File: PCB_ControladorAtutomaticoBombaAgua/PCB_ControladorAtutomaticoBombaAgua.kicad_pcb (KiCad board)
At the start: 4 copper layers, 78 x 57 mm, 20 parts, among them J1 Sensor, K1 Relay12V, K2 Relay12V, P1 12V, P2 230VAC/50Hz, P3 Motor/Bomba, Q1 BC547, Q2 BC547, Q3 BC547, U1 CD4011

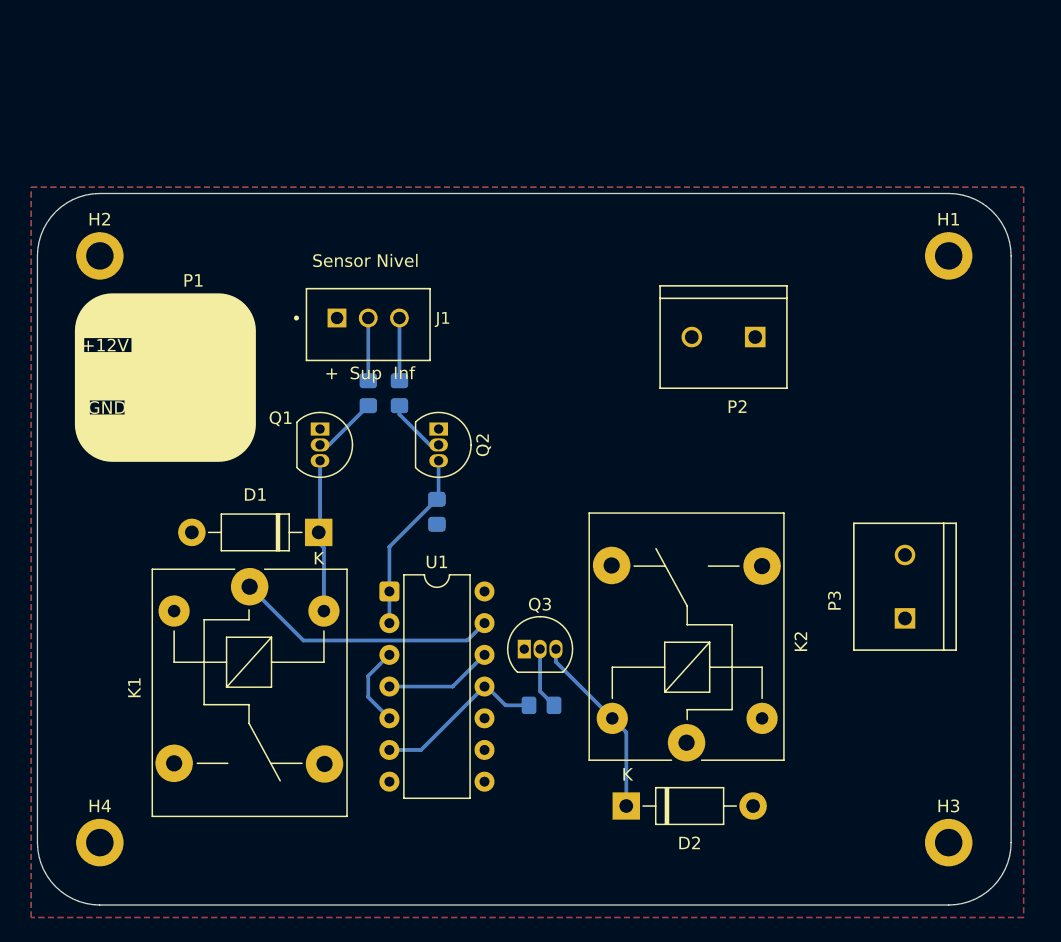
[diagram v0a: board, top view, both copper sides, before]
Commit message: Finalizado
Diseño completado
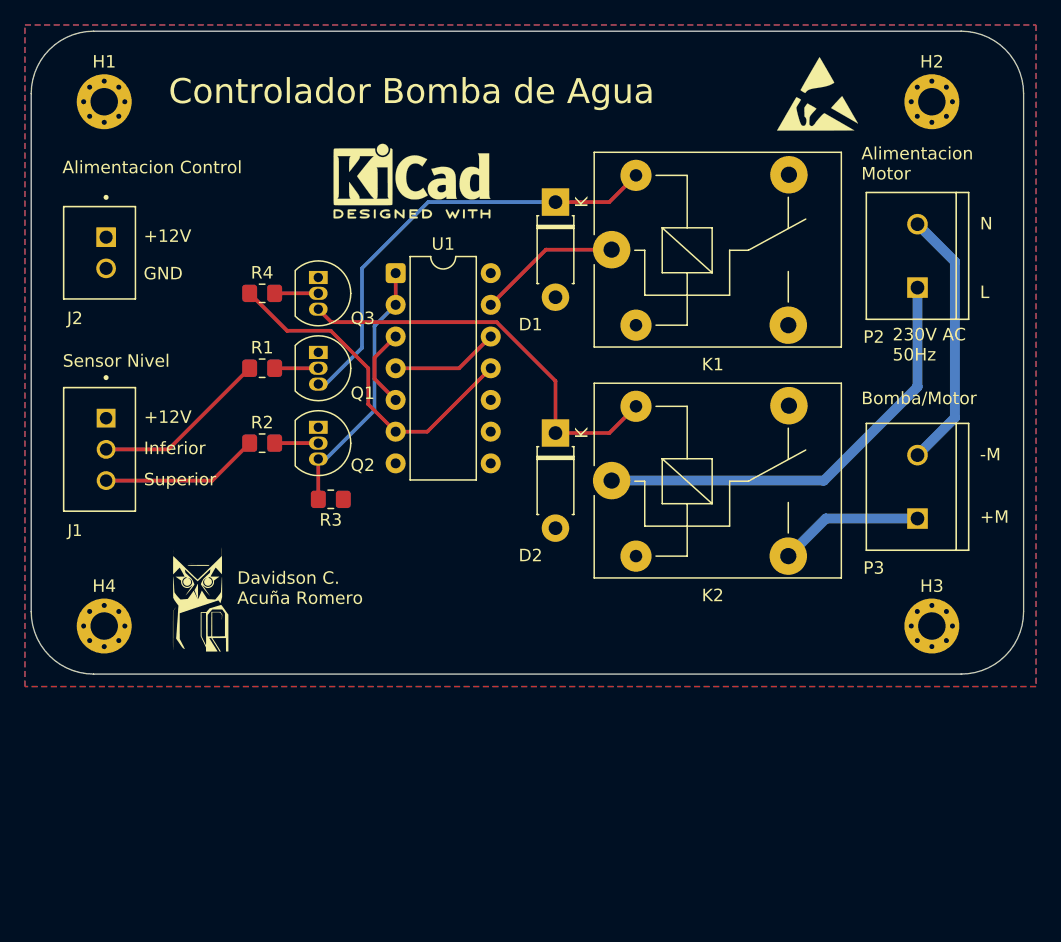
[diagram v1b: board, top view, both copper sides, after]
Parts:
- removed P1: 12V, BORNERA_2:BORNERA-2
- added G***: LOGO, SHIFT:Buho_10X10mm, F.Cu at (135.5, 88.5)
- added G***: LOGO, Huellas:Sensor16x20, B.Cu at (137.0, 66.0)
- added J2: Alimen/Control, JST_XH_2:JST_B2B-XH-A, F.Cu at (127.5, 60.8)
- added REF**: ESD-Logo_6.6x6mm_SilkScreen, Symbol:ESD-Logo_6.6x6mm_SilkScreen, F.Cu at (185.0, 48.0)
- added REF**: KiCad-Logo2_5mm_SilkScreen, Symbol:KiCad-Logo2_5mm_SilkScreen, F.Cu at (152.5, 55.0)
- D1, D2: footprint Diode_THT:D_DO-41_SOD81_P10.16mm_Horizontal -> Diode_THT:D_DO-41_SOD81_P7.62mm_Horizontal
- H1, H2, H3, H4: footprint MountingHole:MountingHole_2.2mm_M2_DIN965_Pad -> MountingHole:MountingHole_2.2mm_M2_Pad_Via
- R1, R2, R3, R4: moved to F.Cu
- moved H1 68.8 mm to (127.8, 48.6)
- moved H2 67.8 mm to (194.2, 48.6)
- moved R4 39.9 mm to (140.5, 64.0)
- moved K1 39.6 mm to (168.5, 60.5), turned to 0 degrees
- moved Q3 34.0 mm to (145.0, 62.7), turned to -90 degrees
- moved D1 32.6 mm to (164.0, 56.7), turned to -90 degrees
- moved D2 30.4 mm to (164.0, 75.2), turned to -90 degrees
- moved U1 25.5 mm to (151.2, 62.4)
- moved J1 23.7 mm to (127.5, 76.5), turned to 90 degrees
- moved K2 21.8 mm to (168.5, 79.0), turned to 0 degrees
- moved H3 17.4 mm to (194.2, 90.7)
- moved H4 17.4 mm to (127.8, 90.7)
- moved P2 16.8 mm to (193.0, 61.0), turned to 90 degrees
- moved R2 11.7 mm to (140.5, 76.0), turned to 0 degrees
- moved Q2 9.64 mm to (145.0, 74.7)
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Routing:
- net LINE: track 0.00 -> 35.6 mm
- net Net-(D1-K): track 12.3 -> 36.1 mm
- net NEUT: track 0.00 -> 21.0 mm
- net Net-(D2-K): track 14.9 -> 32.9 mm
- net Net-(R4-Pad1): track 13.9 -> 27.7 mm
- net Net-(K1-Pad1): track 21.2 -> 11.5 mm
- net /LimiteInferior: track 5.03 -> 14.2 mm
- net /LimiteSuperior: track 5.03 -> 12.7 mm
- net Net-(Q2-E): track 14.6 -> 21.0 mm
- net Net-(Q1-B): track 5.16 -> 3.50 mm
- net Net-(K2-Pad3): track 13.2 -> 11.6 mm
- net Net-(Q3-B): track 4.96 -> 3.50 mm
- net Net-(Q2-B): track 4.85 -> 3.50 mm
- added copper zone on B.Cu, net +12V
- added copper zone on F.Cu, net GND
- removed copper zone on F.Cu, net +12V
- removed copper zone on B.Cu, net GND
- removed copper zone on In1.Cu, net LINE
- removed copper zone on In2.Cu, net NEUT
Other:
- board size 78 x 57 mm -> 79.5 x 51.5 mm
- copper layers 4 -> 2
- board text added: "+M"
- board text added: "-M"
- board text added: "230V AC 50Hz"
- board text added: "Alimentacion Control"
- board text added: "Alimentacion Motor"
- board text added: "Bomba/Motor"
- board text added: "Controlador Bomba de Agua"
- board text added: "Davidson C. Acuña Romero"
- board text added: "Esquema Sensor de Nivel"
- board text added: "Inferior"
- board text added: "L"
- board text added: "N"
- board text added: "Superior"
- board text removed: "+"
- board text removed: "Inf"
- board text removed: "Sup"
